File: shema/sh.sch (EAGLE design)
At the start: 6 parts, among them X1 X1, X2 X2, X3 X3, X4 X4, X5 x5, X6 x6

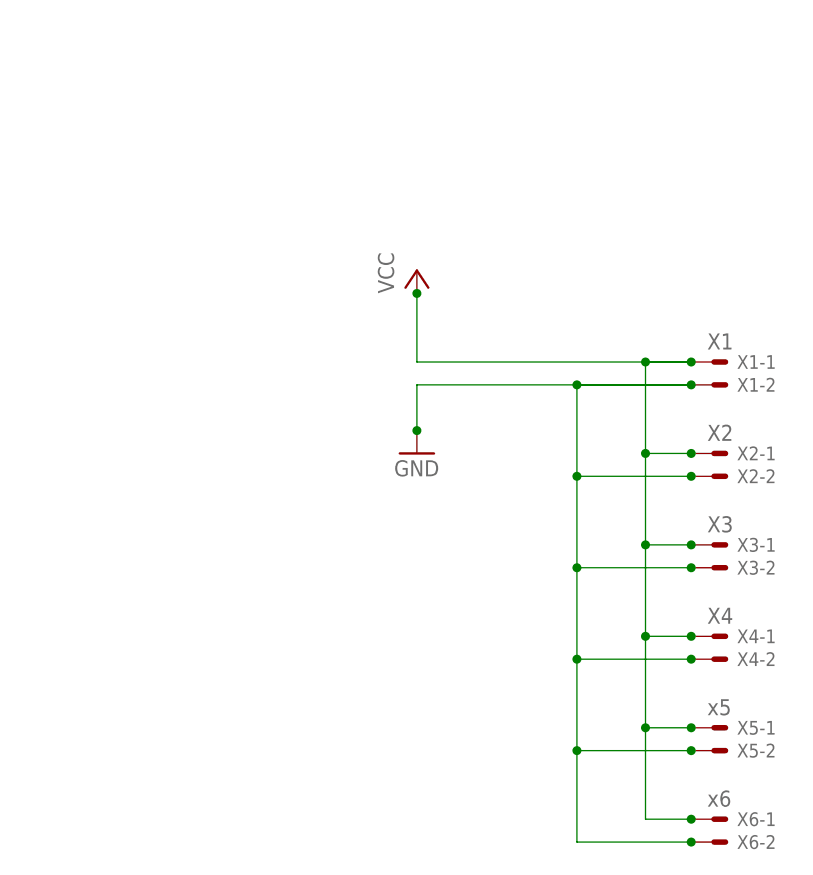
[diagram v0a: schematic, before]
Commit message: ~
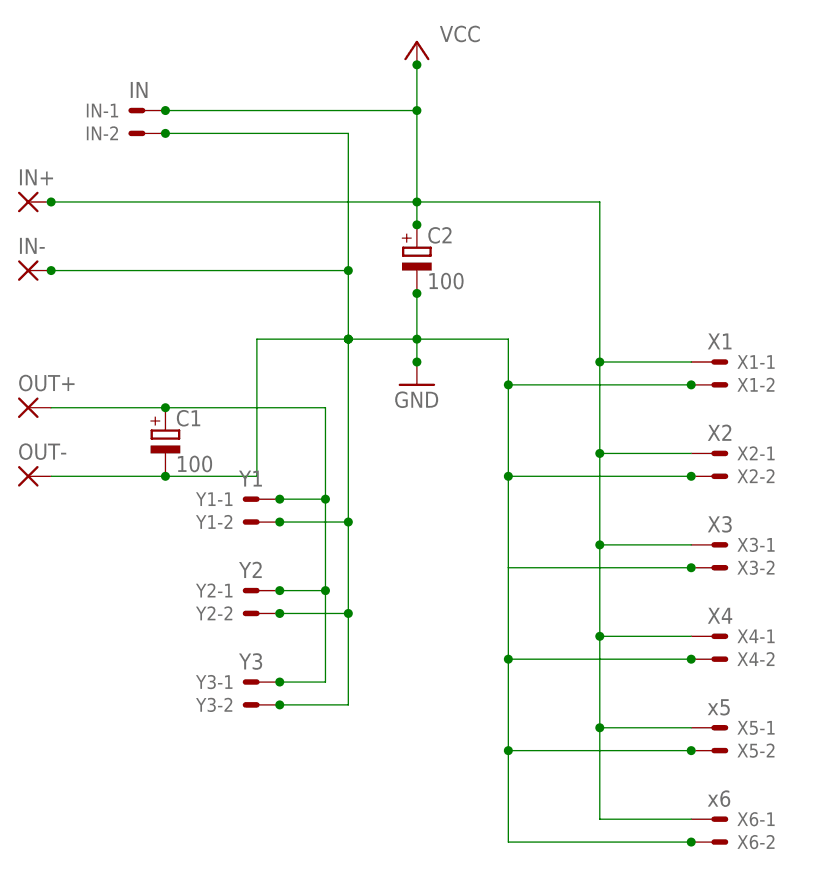
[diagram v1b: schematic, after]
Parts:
- added C1, C2: 100, rcl:CPOL-EUE5-10.5
- added IN: IN, con-molex:C-GRID-02-70543
- added IN+, IN-, OUT+, OUT-: (no value), wirepad:3,17/1,3
- added Y1: Y1, con-molex:C-GRID-02-70543
- added Y2: Y2, con-molex:C-GRID-02-70543
- added Y3: Y3, con-molex:C-GRID-02-70543
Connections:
- new net N$3: C1.+, OUT+.P, Y1-1.S, Y2-1.S, Y3-1.S
- net GND: now also C1.-, C2.-, IN-.P, IN-2.S, OUT-.P, Y1-2.S, Y2-2.S, Y3-2.S
- net VCC: now also C2.+, IN+.P, IN-1.S
